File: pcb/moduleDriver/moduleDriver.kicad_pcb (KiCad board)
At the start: 2 copper layers, 51.4 x 80 mm, 43 parts, among them J1 UART_RL, J10 Sensor, J11 Power, J12 Power, J13 Neopixel, J2 UART_LR, J3 MOTOR, J4 MOTOR, J5 MOTOR, J6 MOTOR, J7 Sensor, J8 Sensor, J9 Sensor, U1 MC7805BDTG, U2 PicoW, U3 ULN2803A, U4 ULN2803A, U5 74HCT2G04GV

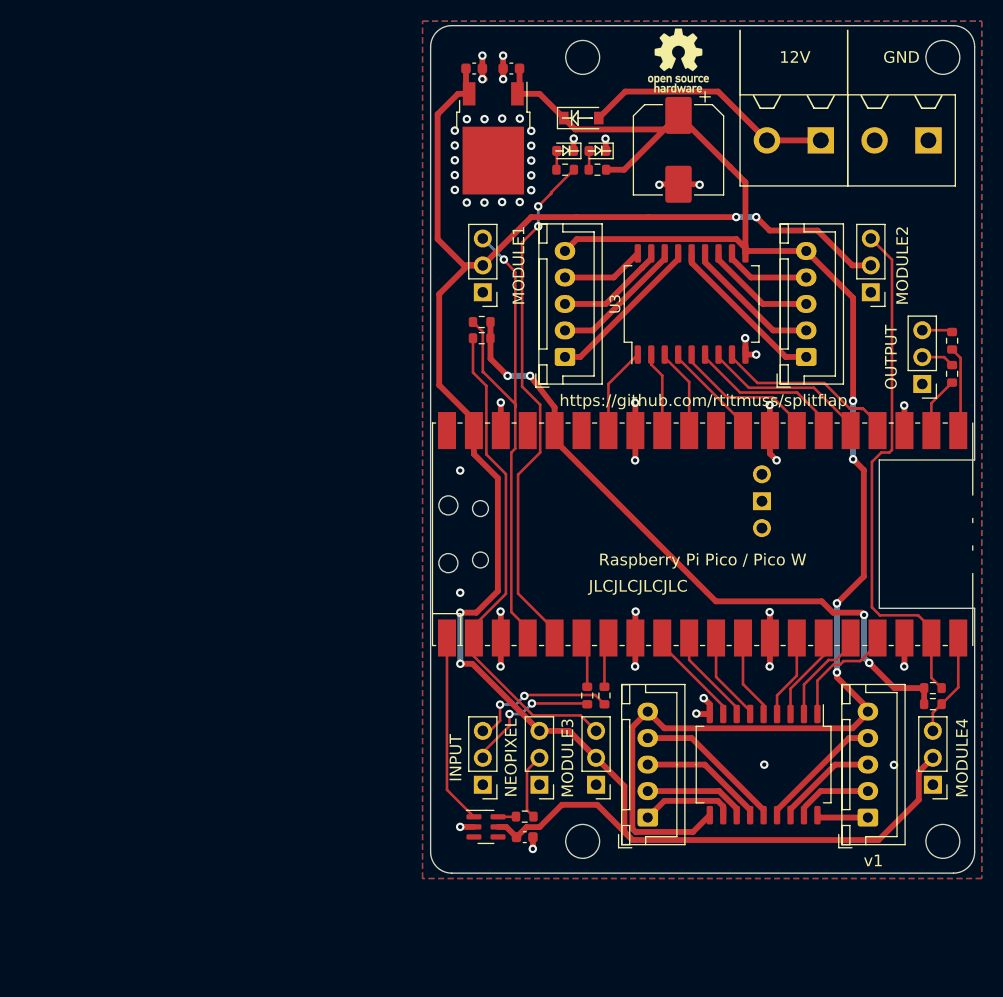
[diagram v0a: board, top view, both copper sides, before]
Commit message: Single thread
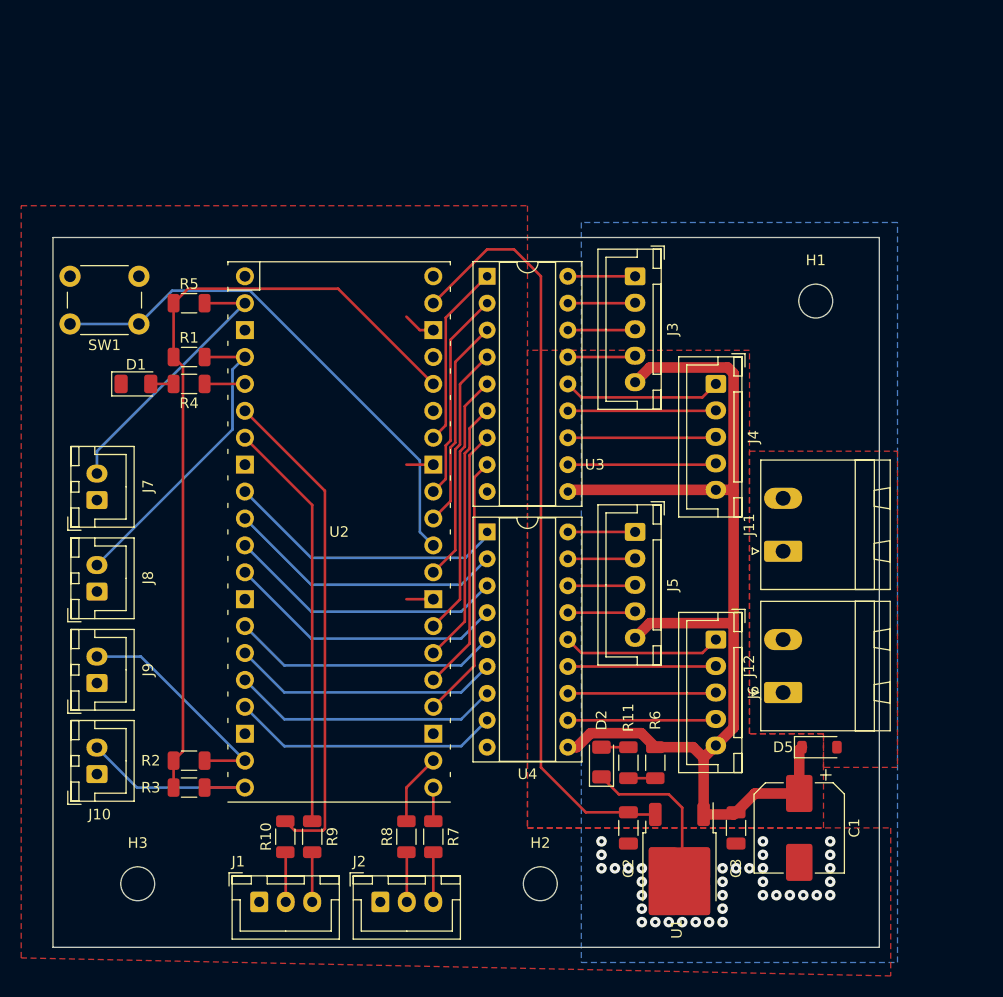
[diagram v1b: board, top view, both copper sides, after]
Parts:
- removed C4: 0.1uF, Capacitor_SMD:C_0603_1608Metric
- removed H4: MountingHole, MountingHole:MountingHole_3.2mm_M3_ISO7380
- removed J13: Neopixel, Connector_PinHeader_2.54mm:PinHeader_1x03_P2.54mm_Vertical
- removed QR*****: github_qrcode, Library:github_qrcode
- removed QR*****: printables_qrcode, Library:printables_qrcode
- removed REF**: OSHW-Logo_5.7x6mm_SilkScreen, Symbol:OSHW-Logo_5.7x6mm_SilkScreen
- removed U5: 74HCT2G04GV, Package_SO:SC-74-6_1.5x2.9mm_P0.95mm
- added SW1: RUN, Button_Switch_THT:SW_PUSH_6mm, F.Cu at (61.1, 78.2)
- added kibuzzard-64922CB7: G***, kibuzzard-64922CB7, B.Cu at (86.4, 127.6)
- added kibuzzard-64922CB7: G***, kibuzzard-64922CB7, B.Cu at (74.9, 127.6)
- added kibuzzard-64922CEC: G***, kibuzzard-64922CEC, B.Cu at (88.9, 127.6)
- added kibuzzard-64922CEC: G***, kibuzzard-64922CEC, B.Cu at (77.5, 127.6)
- C2, C3: footprint Capacitor_SMD:C_0603_1608Metric -> Capacitor_SMD:C_1206_3216Metric
- D1, D2: footprint LED_SMD:LED_0603_1608Metric -> LED_SMD:LED_1206_3216Metric
- J1, J2: footprint Connector_PinHeader_2.54mm:PinHeader_1x03_P2.54mm_Vertical -> Connector_JST:JST_XH_B3B-XH-A_1x03_P2.50mm_Vertical
- J10: value Sensor -> Sense D; footprint Connector_PinHeader_2.54mm:PinHeader_1x03_P2.54mm_Vertical -> Connector_JST:JST_XH_B2B-XH-A_1x02_P2.50mm_Vertical
- J11, J12: footprint Library:ScrewTerminal-5.08-2P -> Connector_Phoenix_MSTB:PhoenixContact_MSTBA_2,5_2-G_1x02_P5.00mm_Horizontal
- J3: value MOTOR -> MOTOR A
- J4: value MOTOR -> MOTOR B
- J5: value MOTOR -> MOTOR C
- J6: value MOTOR -> MOTOR D
- J7: value Sensor -> Sense A; footprint Connector_PinHeader_2.54mm:PinHeader_1x03_P2.54mm_Vertical -> Connector_JST:JST_XH_B2B-XH-A_1x02_P2.50mm_Vertical
- J8: value Sensor -> Sense B; footprint Connector_PinHeader_2.54mm:PinHeader_1x03_P2.54mm_Vertical -> Connector_JST:JST_XH_B2B-XH-A_1x02_P2.50mm_Vertical
- J9: value Sensor -> Sense C; footprint Connector_PinHeader_2.54mm:PinHeader_1x03_P2.54mm_Vertical -> Connector_JST:JST_XH_B2B-XH-A_1x02_P2.50mm_Vertical
- R1, R10, R2, R3, R4, R5, R7, R8, R9: footprint Resistor_SMD:R_0603_1608Metric -> Resistor_SMD:R_1206_3216Metric
- R11: value 470 -> 1.2k; footprint Resistor_SMD:R_0603_1608Metric -> Resistor_SMD:R_1206_3216Metric
- R6: value 2.2k -> 1.2k; footprint Resistor_SMD:R_0603_1608Metric -> Resistor_SMD:R_1206_3216Metric
- U3, U4: footprint Package_SO:SOP-18_7x12.5mm_P1.27mm -> Package_DIP:DIP-18_W7.62mm_Socket
- moved R5 79.1 mm to (65.8, 76.2)
- moved J10 78.9 mm to (57.1, 120.7), turned to 90 degrees
- moved H3 76.1 mm to (61.0, 131.0)
- moved J7 75.6 mm to (57.1, 94.8), turned to 90 degrees
- moved C3 74.8 mm to (117.5, 125.7), turned to -90 degrees
- moved C2 73.1 mm to (107.3, 125.7), turned to -90 degrees
- moved U1 71.1 mm to (112.1, 129.5)
- moved J2 70.8 mm to (83.9, 132.7), turned to 0 degrees
- moved R3 70.6 mm to (65.8, 121.9)
- moved R7 67.7 mm to (88.9, 126.6), turned to 90 degrees
- moved R8 67.5 mm to (86.4, 126.6), turned to 90 degrees
- moved C1 65.0 mm to (123.4, 125.7)
- moved D5 63.5 mm to (125.3, 118.1)
- moved D2 57.7 mm to (104.8, 119.5), turned to 90 degrees
- moved R6 56.2 mm to (109.9, 119.6), turned to -90 degrees
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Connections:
- D2 pad 2: Net-(D2-Pad2) -> Net-(D2-A)
- D5 pad 2: Net-(D5-Pad2) -> VCC
- J10 pad 2: +5V -> /SENSOR_D
- J11 pad 1: Net-(D5-Pad2) -> GND
- J11 pad 2: Net-(D5-Pad2) -> VCC
- J12 pad 2: GND -> VCC
- J7 pad 2: +5V -> /SENSOR_A
- J8 pad 2: +5V -> /SENSOR_B
- J9 pad 2: +5V -> /SENSOR_C
- R11 pad 2: Net-(J13-Pad2) -> Net-(D2-A)
- R6 pad 2: Net-(D2-Pad2) -> Net-(R11-Pad1)
- U2 pad 1: /NEOPIXEL -> unconnected-(U2-GPIO0/TX0-Pad1)
- U2 pad 10: /MOTOR_D_PHASE_C_P -> /MOTOR_C_PHASE_B_P
- U2 pad 11: /MOTOR_D_PHASE_B_P -> /MOTOR_C_PHASE_C_P
- U2 pad 12: /MOTOR_D_PHASE_A_P -> /MOTOR_C_PHASE_D_P
- U2 pad 14: /MOTOR_C_PHASE_D_P -> /MOTOR_D_PHASE_A_P
- U2 pad 15: /MOTOR_C_PHASE_C_P -> /MOTOR_D_PHASE_B_P
- U2 pad 16: /MOTOR_C_PHASE_B_P -> /MOTOR_D_PHASE_C_P
- U2 pad 17: /MOTOR_C_PHASE_A_P -> /MOTOR_D_PHASE_D_P
- U2 pad 19: /SENSOR_A -> /SENSOR_C
- U2 pad 2: /SENSOR_C -> /SENSOR_A
- U2 pad 30: unconnected-(U2-Pad30) -> /RUN
- U2 pad 9: /MOTOR_D_PHASE_D_P -> /MOTOR_C_PHASE_A_P
- U3 pad 15: /MOTOR_A_PHASE_A -> /MOTOR_A_PHASE_D
- U3 pad 16: /MOTOR_A_PHASE_B -> /MOTOR_A_PHASE_C
- U3 pad 17: /MOTOR_A_PHASE_C -> /MOTOR_A_PHASE_B
- U3 pad 18: /MOTOR_A_PHASE_D -> /MOTOR_A_PHASE_A
- U4 pad 11: /MOTOR_D_PHASE_A -> /MOTOR_D_PHASE_D
- U4 pad 12: /MOTOR_D_PHASE_B -> /MOTOR_D_PHASE_C
- U4 pad 13: /MOTOR_D_PHASE_C -> /MOTOR_D_PHASE_B
- U4 pad 14: /MOTOR_D_PHASE_D -> /MOTOR_D_PHASE_A
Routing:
- net +5V: track 181.2 -> 72.3 mm, vias 4 -> 0
- net +12V: track 158.5 -> 107.3 mm, vias 4 -> 0
- net /RUN: track 0.00 -> 49.5 mm
- net /LED: track 48.3 -> 3.81 mm, vias 2 -> 0
- net /UART_RL_TX: track 5.73 -> 46.8 mm
- net /UART_RL_RX: track 5.66 -> 38.8 mm
- net GND: track 55.6 -> 23.3 mm, vias 49 -> 36
- net /SENSOR_C: track 46.8 -> 21.9 mm
- net Net-(D5-Pad2): track 23.9 -> 0.00 mm
- net /SENSOR_A: track 49.3 -> 25.7 mm
- net /SENSOR_B: track 48.5 -> 29.2 mm, vias 1 -> 0
- net /NEOPIXEL: track 18.8 -> 0.00 mm
- net /MOTOR_C_PHASE_B_P: track 8.71 -> 26.5 mm
- net /MOTOR_C_PHASE_D_P: track 8.85 -> 26.5 mm
- net /MOTOR_D_PHASE_D_P: track 8.14 -> 25.4 mm
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- added copper zone on F.Cu, net +12V
- added copper zone on F.Cu, net VCC
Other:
- board size 51.4 x 80 mm -> 78 x 67 mm
- board text removed: "12V"
- board text removed: "Designed for https://www.printables.com/ model/69464-split-flap-display by David Kingsman"
- board text removed: "GND"
- board text removed: "INPUT"
- board text removed: "JLCJLCJLCJLC"
- board text removed: "MODULE1"
- board text removed: "MODULE2"
- board text removed: "MODULE3"
- board text removed: "MODULE4"
- board text removed: "NEOPIXEL"
- board text removed: "OUTPUT"
- board text removed: "Raspberry Pi Pico / Pico W"
- board text removed: "https://github.com/rtitmuss/splitflap"
- board text removed: "v1"
